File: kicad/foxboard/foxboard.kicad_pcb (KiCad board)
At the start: 2 copper layers, 356.7 x 154.4 mm, 183 parts, among them J2 USB_C_Receptacle_USB2.0, K1 KEYSW, K10 KEYSW, K11 KEYSW, K12 KEYSW, K13 KEYSW, K14 KEYSW, K15 KEYSW, K16 KEYSW, K17 KEYSW, K18 KEYSW, K19 KEYSW, K2 KEYSW, K20 KEYSW, K21 KEYSW, K22 KEYSW, K23 KEYSW, K24 KEYSW, K25 KEYSW, K26 KEYSW, K27 KEYSW, K28 KEYSW, K29 KEYSW, K3 KEYSW, K30 KEYSW, K31 KEYSW, K32 KEYSW, K33 KEYSW, K34 KEYSW, K35 KEYSW, K36 KEYSW, K37 KEYSW, K38 KEYSW, K39 KEYSW, K4 KEYSW, K40 KEYSW, K41 KEYSW, K42 KEYSW, K43 KEYSW, K44 KEYSW, K45 KEYSW, K46 KEYSW, K47 KEYSW, K48 KEYSW, K49 KEYSW, K5 KEYSW, K50 KEYSW, K51 KEYSW, K52 KEYSW, K53 KEYSW, K54 KEYSW, K55 KEYSW, K56 KEYSW, K57 KEYSW, K58 KEYSW, K59 KEYSW, K6 KEYSW, K60 KEYSW, K61 KEYSW, K62 KEYSW, K63 KEYSW, K64 KEYSW, K65 KEYSW, K66 KEYSW, K67 KEYSW, K68 KEYSW, K69 KEYSW, K7 KEYSW, K70 KEYSW, K71 KEYSW, K72 KEYSW, K73 KEYSW, K74 KEYSW, K75 KEYSW, K76 KEYSW, K77 KEYSW, K78 KEYSW, K79 KEYSW, K8 KEYSW, K80 KEYSW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

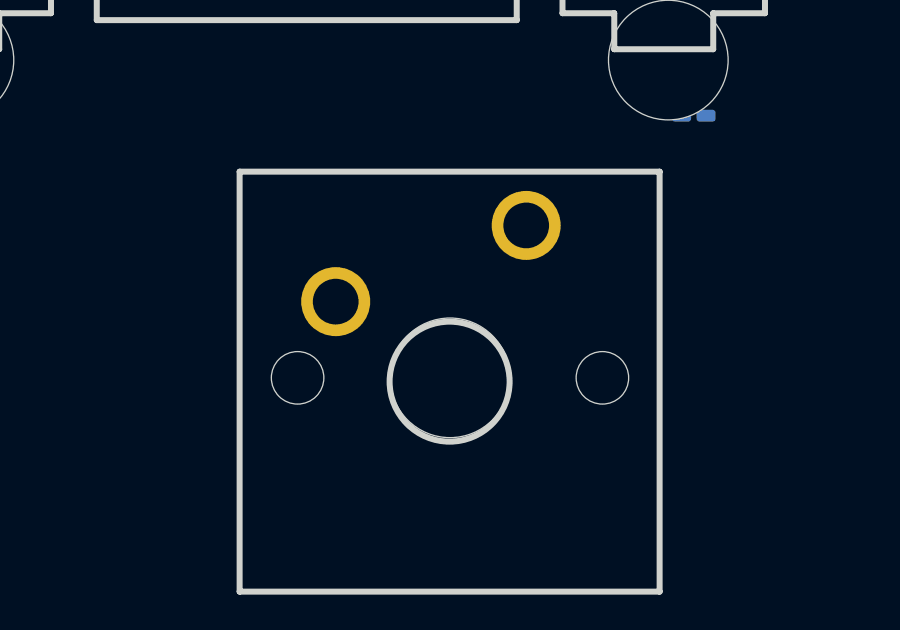
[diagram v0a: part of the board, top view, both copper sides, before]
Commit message: update footprint to be 1.5u
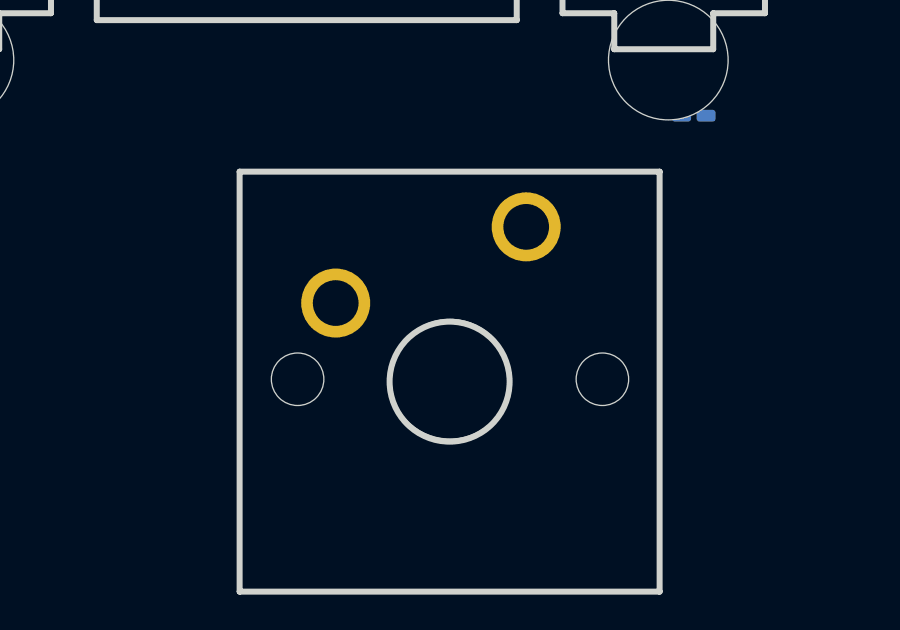
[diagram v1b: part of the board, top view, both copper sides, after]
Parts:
- K51: footprint PCM_marbastlib-mx:SW_MX_1.25u -> PCM_marbastlib-mx:SW_MX_1.5u
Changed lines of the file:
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@@
       (net 85 "Net-(D77-A)") (pintype "passive"))
   )
-  (footprint "PCM_marbastlib-mx:SW_MX_1.25u" (layer "F.Cu")
-    (at 248.08785 286.9726)
+  (footprint "PCM_marbastlib-mx:SW_MX_1.5u" (layer "F.Cu")
+    (at 248.08785 287.02)
     (descr "Footprint for Cherry MX style switches")
     (property "Sheetfile" "foxboard.kicad_sch")
     (property "Sheetname" "")
-    (attr through_hole exclude_from_pos_files)
+    (attr through_hole exclude_from_pos_files exclude_from_bom)
     (fp_text reference "K51" (at 0 3.175) (layer "Dwgs.User") hide
         (effects (font (size 1 1) (thickness 0.15)))
@@
         (effects (font (size 1 1) (thickness 0.15)))
     )
-    (fp_line (start -11.90625 -9.525) (end -11.90625 9.525)
+    (fp_line (start -14.2875 -9.525) (end -14.2875 9.525)
       (stroke (width 0.12) (type solid)) (layer "Dwgs.User"))
-    (fp_line (start -11.90625 9.525) (end 11.90625 9.525)
+    (fp_line (start -14.2875 9.525) (end 14.2875 9.525)
       (stroke (width 0.12) (type solid)) (layer "Dwgs.User"))
-    (fp_line (start 11.90625 -9.525) (end -11.90625 -9.525)
+    (fp_line (start 14.2875 -9.525) (end -14.2875 -9.525)
       (stroke (width 0.12) (type solid)) (layer "Dwgs.User"))
-    (fp_line (start 11.90625 9.525) (end 11.90625 -9.525)
+    (fp_line (start 14.2875 9.525) (end 14.2875 -9.525)
       (stroke (width 0.12) (type solid)) (layer "Dwgs.User"))
     (fp_line (start -7 6.5) (end -7 -6.5)
